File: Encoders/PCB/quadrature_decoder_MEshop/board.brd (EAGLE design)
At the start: 84.8 x 55.9 mm, 14 parts, among them IC1 LFLS7366R, IC2 LFLS7366R, IC3 LFLS7366R, IC4 LFLS7366R, IC5 LFLS7366R, IC6 LFLS7366R

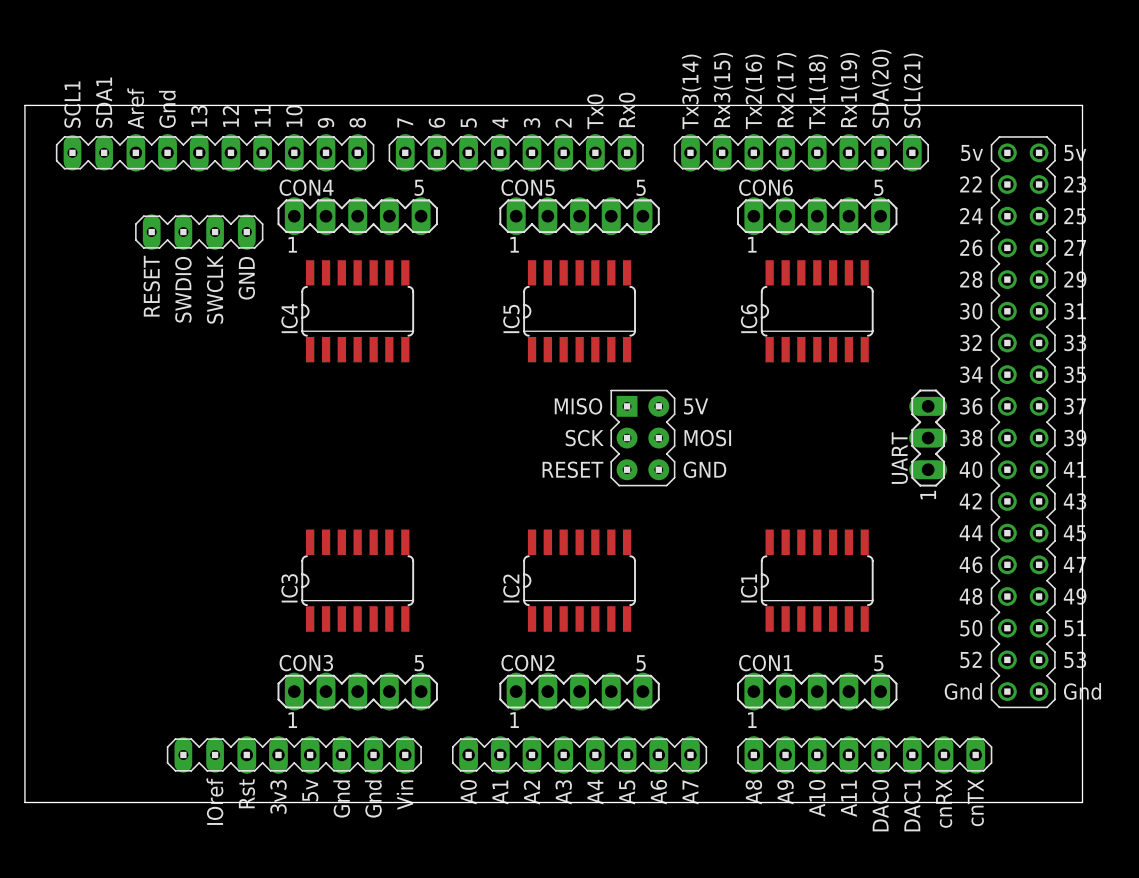
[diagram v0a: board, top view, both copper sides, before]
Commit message: new boards and stuff
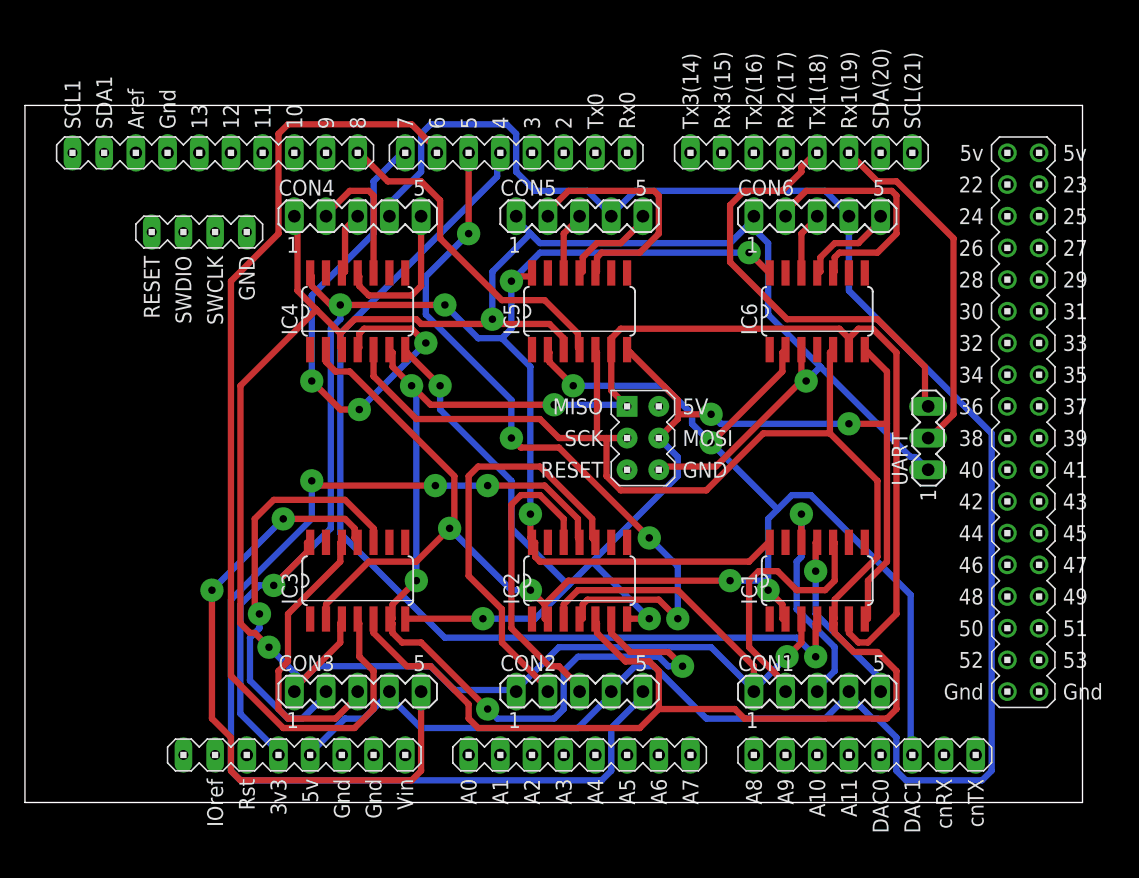
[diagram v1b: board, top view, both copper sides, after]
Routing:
- net GND: track 0.00 -> 221.1 mm, vias 0 -> 4
- net 5V: track 0.00 -> 165.9 mm
- net SCK: track 0.00 -> 148.7 mm
- net MISO: track 0.00 -> 139.5 mm, vias 0 -> 5
- net FCKI: track 0.00 -> 135.0 mm, vias 0 -> 6
- net 3.3V: track 0.00 -> 131.7 mm, vias 0 -> 6
- net MOSI: track 0.00 -> 112.5 mm, vias 0 -> 5
- net N$7: track 0.00 -> 89.0 mm, vias 0 -> 3
- net SS1: track 0.00 -> 81.2 mm, vias 0 -> 1
- net SS3: track 0.00 -> 81.0 mm
- net SS2: track 0.00 -> 58.7 mm, vias 0 -> 4
- net N$10: track 0.00 -> 52.6 mm, vias 0 -> 2
- net SS4: track 0.00 -> 41.1 mm, vias 0 -> 3
- net N$3: track 0.00 -> 35.9 mm
- net N$8: track 0.00 -> 34.0 mm, vias 0 -> 1
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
